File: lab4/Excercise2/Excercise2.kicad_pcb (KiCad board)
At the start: 2 copper layers, 30.5 x 38.1 mm, 10 parts, among them J1 Conn_01x02_Male, U1 NE555D

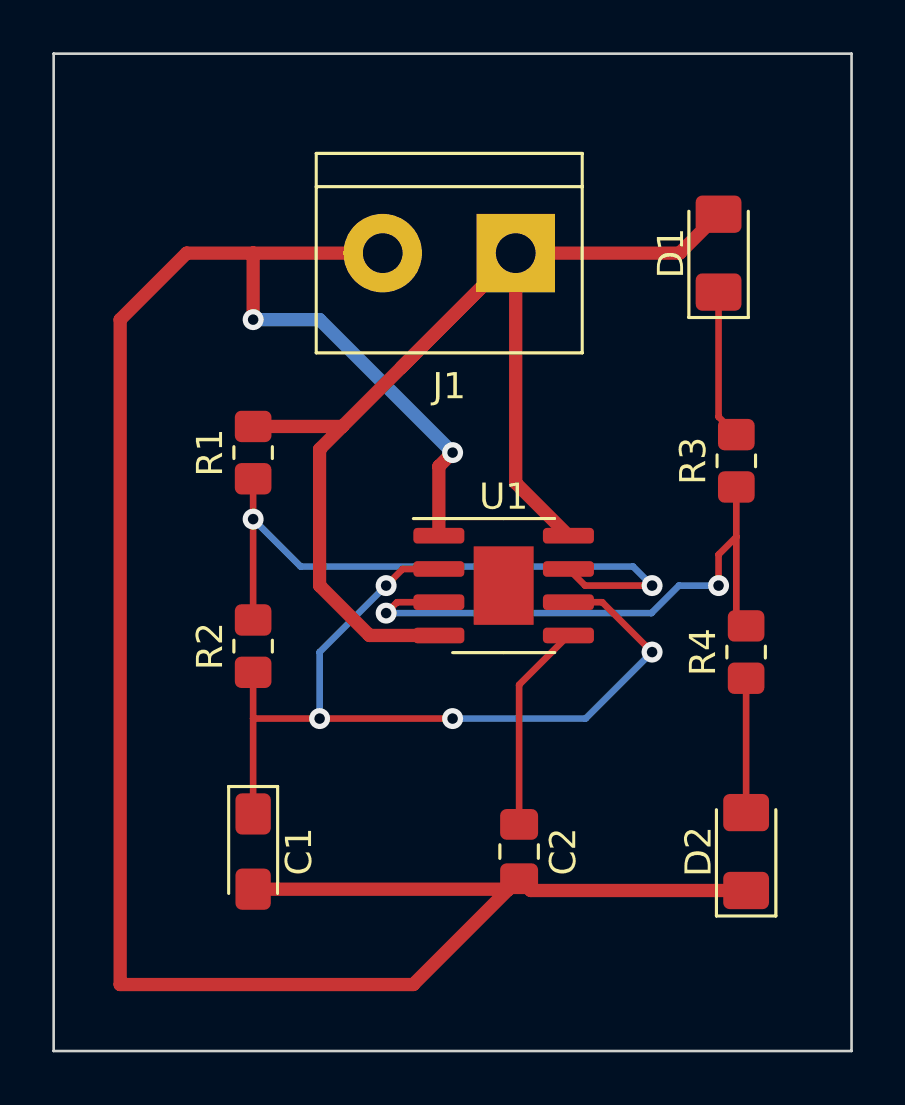
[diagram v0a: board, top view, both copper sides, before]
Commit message: Generated Gerber files
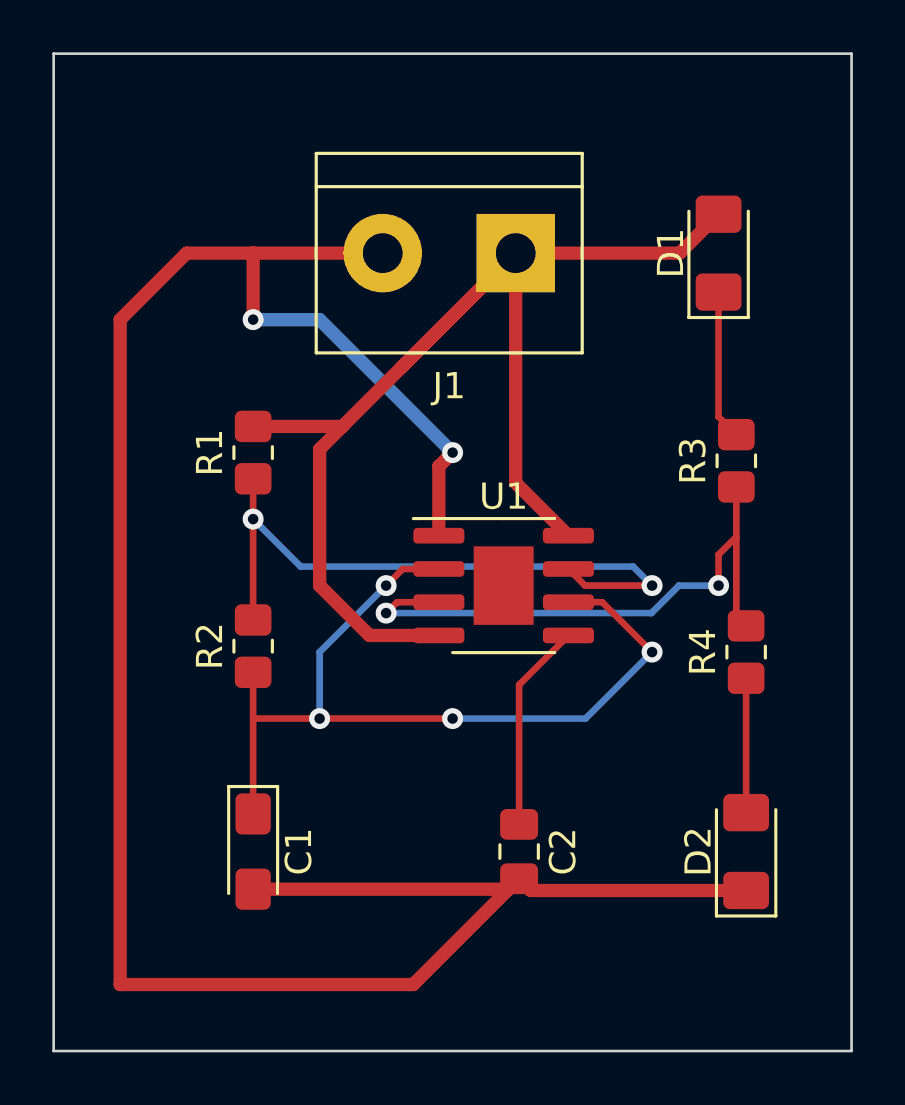
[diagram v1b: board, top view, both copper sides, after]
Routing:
- added copper zone on B.Cu, net GND
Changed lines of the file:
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@@
       (outputformat 1)
       (mirror false)
-      (drillshape 1)
+      (drillshape 0)
       (scaleselection 1)
-      (outputdirectory "")
+      (outputdirectory "output files/")
     )
   )
@@
     (fp_line (start 1.6 0.8) (end 1.6 -0.8) (layer "F.Fab") (width 0.1))
     (fp_line (start 1.6 -0.8) (end -1.2 -0.8) (layer "F.Fab") (width 0.1))
-    (pad "1" smd roundrect (at -1.4875 0 90) (size 1.425 1.75) (layers "F.Cu" "F.Paste" "F.Mask") (roundrect_rratio 0.175439)
+    (pad "1" smd roundrect (at -1.4875 0 90) (size 1.425 1.75) (layers "F.Cu" "F.Paste" "F.Mask") (roundrect_rratio 0.1754392982)
       (net 4 "Net-(D1-Pad1)") (pinfunction "K") (pintype "passive"))
-    (pad "2" smd roundrect (at 1.4875 0 90) (size 1.425 1.75) (layers "F.Cu" "F.Paste" "F.Mask") (roundrect_rratio 0.175439)
+    (pad "2" smd roundrect (at 1.4875 0 90) (size 1.425 1.75) (layers "F.Cu" "F.Paste" "F.Mask") (roundrect_rratio 0.1754392982)
       (net 5 "+9V") (pinfunction "A") (pintype "passive"))
     (model "${KICAD6_3DMODEL_DIR}/LED_SMD.3dshapes/LED_1206_3216Metric.wrl"
@@
     (fp_line (start 1 -0.625) (end 1 0.625) (layer "F.Fab") (width 0.1))
     (fp_line (start 1 0.625) (end -1 0.625) (layer "F.Fab") (width 0.1))
-    (pad "1" smd roundrect (at -1 0 90) (size 1.2 1.4) (layers "F.Cu" "F.Paste" "F.Mask") (roundrect_rratio 0.208333)
+    (pad "1" smd roundrect (at -1 0 90) (size 1.2 1.4) (layers "F.Cu" "F.Paste" "F.Mask") (roundrect_rratio 0.2083333333)
       (net 1 "/pin_2") (pintype "passive"))
-    (pad "2" smd roundrect (at 1 0 90) (size 1.2 1.4) (layers "F.Cu" "F.Paste" "F.Mask") (roundrect_rratio 0.208333)
+    (pad "2" smd roundrect (at 1 0 90) (size 1.2 1.4) (layers "F.Cu" "F.Paste" "F.Mask") (roundrect_rratio 0.2083333333)
       (net 7 "/pin_7") (pintype "passive"))
     (model "${KICAD6_3DMODEL_DIR}/Resistor_SMD.3dshapes/R_0805_2012Metric.wrl"
@@
     (fp_line (start 1.6 0.8) (end 1.6 -0.8) (layer "F.Fab") (width 0.1))
     (fp_line (start -1.6 0.8) (end 1.6 0.8) (layer "F.Fab") (width 0.1))
-    (pad "1" smd roundrect (at -1.4375 0 270) (size 1.575 1.35) (layers "F.Cu" "F.Paste" "F.Mask") (roundrect_rratio 0.185185)
+    (pad "1" smd roundrect (at -1.4375 0 270) (size 1.575 1.35) (layers "F.Cu" "F.Paste" "F.Mask") (roundrect_rratio 0.1851851852)
       (net 1 "/pin_2") (pintype "passive"))
-    (pad "2" smd roundrect (at 1.4375 0 270) (size 1.575 1.35) (layers "F.Cu" "F.Paste" "F.Mask") (roundrect_rratio 0.185185)
+    (pad "2" smd roundrect (at 1.4375 0 270) (size 1.575 1.35) (layers "F.Cu" "F.Paste" "F.Mask") (roundrect_rratio 0.1851851852)
       (net 2 "GND") (pintype "passive"))
     (model "${KICAD6_3DMODEL_DIR}/Capacitor_Tantalum_SMD.3dshapes/CP_EIA-3216-18_Kemet-A.wrl"
@@
     (fp_line (start 1 0.625) (end -1 0.625) (layer "F.Fab") (width 0.1))
     (fp_line (start -1 0.625) (end -1 -0.625) (layer "F.Fab") (width 0.1))
-    (pad "1" smd roundrect (at -1 0 90) (size 1.2 1.4) (layers "F.Cu" "F.Paste" "F.Mask") (roundrect_rratio 0.208333)
+    (pad "1" smd roundrect (at -1 0 90) (size 1.2 1.4) (layers "F.Cu" "F.Paste" "F.Mask") (roundrect_rratio 0.2083333333)
       (net 6 "Net-(D2-Pad2)") (pintype "passive"))
-    (pad "2" smd roundrect (at 1 0 90) (size 1.2 1.4) (layers "F.Cu" "F.Paste" "F.Mask") (roundrect_rratio 0.208333)
+    (pad "2" smd roundrect (at 1 0 90) (size 1.2 1.4) (layers "F.Cu" "F.Paste" "F.Mask") (roundrect_rratio 0.2083333333)
       (net 8 "/pin_3") (pintype "passive"))
     (model "${KICAD6_3DMODEL_DIR}/Resistor_SMD.3dshapes/R_0805_2012Metric.wrl"
@@
     (fp_line (start -1 -0.625) (end 1 -0.625) (layer "F.Fab") (width 0.1))
     (fp_line (start 1 0.625) (end -1 0.625) (layer "F.Fab") (width 0.1))
-    (pad "1" smd roundrect (at -1.0375 0 270) (size 1.175 1.45) (layers "F.Cu" "F.Paste" "F.Mask") (roundrect_rratio 0.212766)
+    (pad "1" smd roundrect (at -1.0375 0 270) (size 1.175 1.45) (layers "F.Cu" "F.Paste" "F.Mask") (roundrect_rratio 0.2127659574)
       (net 3 "Net-(C2-Pad1)") (pintype "passive"))
-    (pad "2" smd roundrect (at 1.0375 0 270) (size 1.175 1.45) (layers "F.Cu" "F.Paste" "F.Mask") (roundrect_rratio 0.212766)
+    (pad "2" smd roundrect (at 1.0375 0 270) (size 1.175 1.45) (layers "F.Cu" "F.Paste" "F.Mask") (roundrect_rratio 0.2127659574)
       (net 2 "GND") (pintype "passive"))
     (model "${KICAD6_3DMODEL_DIR}/Capacitor_SMD.3dshapes/C_0805_2012Metric.wrl"
@@
     (fp_line (start 1 0.625) (end -1 0.625) (layer "F.Fab") (width 0.1))
     (fp_line (start -1 0.625) (end -1 -0.625) (layer "F.Fab") (width 0.1))
-    (pad "1" smd roundrect (at -1 0 90) (size 1.2 1.4) (layers "F.Cu" "F.Paste" "F.Mask") (roundrect_rratio 0.208333)
+    (pad "1" smd roundrect (at -1 0 90) (size 1.2 1.4) (layers "F.Cu" "F.Paste" "F.Mask") (roundrect_rratio 0.2083333333)
       (net 8 "/pin_3") (pintype "passive"))
-    (pad "2" smd roundrect (at 1 0 90) (size 1.2 1.4) (layers "F.Cu" "F.Paste" "F.Mask") (roundrect_rratio 0.208333)
+    (pad "2" smd roundrect (at 1 0 90) (size 1.2 1.4) (layers "F.Cu" "F.Paste" "F.Mask") (roundrect_rratio 0.2083333333)
       (net 4 "Net-(D1-Pad1)") (pintype "passive"))
     (model "${KICAD6_3DMODEL_DIR}/Resistor_SMD.3dshapes/R_0805_2012Metric.wrl"
@@
     (fp_line (start 1 -0.625) (end 1 0.625) (layer "F.Fab") (width 0.1))
     (fp_line (start -1 -0.625) (end 1 -0.625) (layer "F.Fab") (width 0.1))
-    (pad "1" smd roundrect (at -1 0 90) (size 1.2 1.4) (layers "F.Cu" "F.Paste" "F.Mask") (roundrect_rratio 0.208333)
+    (pad "1" smd roundrect (at -1 0 90) (size 1.2 1.4) (layers "F.Cu" "F.Paste" "F.Mask") (roundrect_rratio 0.2083333333)
       (net 7 "/pin_7") (pintype "passive"))
-    (pad "2" smd roundrect (at 1 0 90) (size 1.2 1.4) (layers "F.Cu" "F.Paste" "F.Mask") (roundrect_rratio 0.208333)
+    (pad "2" smd roundrect (at 1 0 90) (size 1.2 1.4) (layers "F.Cu" "F.Paste" "F.Mask") (roundrect_rratio 0.2083333333)
       (net 5 "+9V") (pintype "passive"))
     (model "${KICAD6_3DMODEL_DIR}/Resistor_SMD.3dshapes/R_0805_2012Metric.wrl"
@@
     (fp_line (start -1.6 -0.4) (end -1.6 0.8) (layer "F.Fab") (width 0.1))
     (fp_line (start -1.2 -0.8) (end -1.6 -0.4) (layer "F.Fab") (width 0.1))
-    (pad "1" smd roundrect (at -1.4875 0 90) (size 1.425 1.75) (layers "F.Cu" "F.Paste" "F.Mask") (roundrect_rratio 0.175439)
+    (pad "1" smd roundrect (at -1.4875 0 90) (size 1.425 1.75) (layers "F.Cu" "F.Paste" "F.Mask") (roundrect_rratio 0.1754392982)
       (net 2 "GND") (pinfunction "K") (pintype "passive"))
-    (pad "2" smd roundrect (at 1.4875 0 90) (size 1.425 1.75) (layers "F.Cu" "F.Paste" "F.Mask") (roundrect_rratio 0.175439)
+    (pad "2" smd roundrect (at 1.4875 0 90) (size 1.425 1.75) (layers "F.Cu" "F.Paste" "F.Mask") (roundrect_rratio 0.1754392982)
       (net 6 "Net-(D2-Pad2)") (pinfunction "A") (pintype "passive"))
     (model "${KICAD6_3DMODEL_DIR}/LED_SMD.3dshapes/LED_1206_3216Metric.wrl"
@@
   (segment (start 157.456634 74.7115) (end 158.508134 73.66) (width 0.254) (layer "B.Cu") (net 8))
   (segment (start 147.32 74.7115) (end 157.456634 74.7115) (width 0.254) (layer "B.Cu") (net 8))
+  (zone (net 2) (net_name "GND") (layer "B.Cu") (hatch edge 0.508)
+    (connect_pads (clearance 0.508))
+    (min_thickness 0.254) (filled_areas_thickness no)
+    (fill yes (thermal_gap 0.508) (thermal_bridge_width 0.508))
+    (polygon
+      (pts
+        (xy 165.1 91.44)
+        (xy 134.62 91.44)
+        (xy 134.62 53.34)
+        (xy 165.1 53.34)
+      )
+    )
+  )
 )
